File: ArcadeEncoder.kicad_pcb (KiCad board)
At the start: 2 copper layers, 56.6 x 38.7 mm, 7 parts, among them J2 DB9_Male, U1 ProMicro

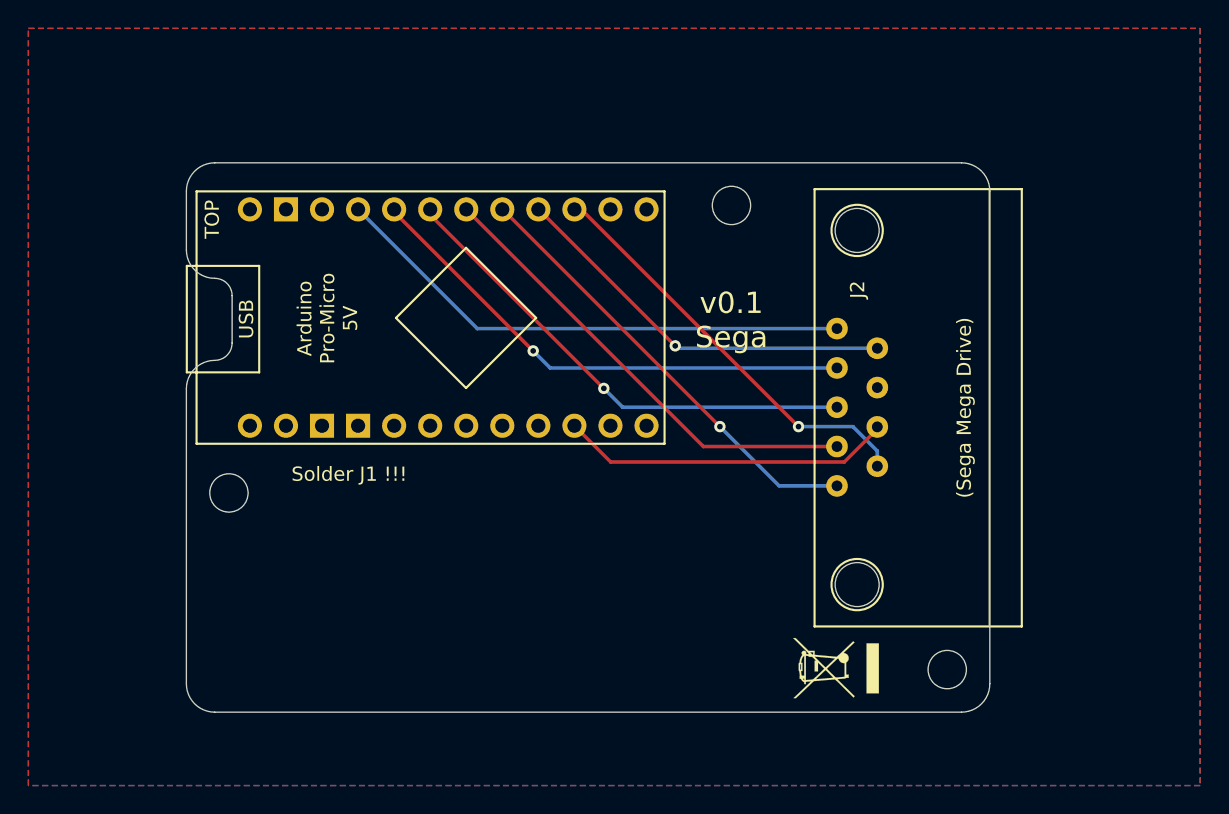
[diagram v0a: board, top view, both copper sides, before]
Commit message: Updated to KiCad 6
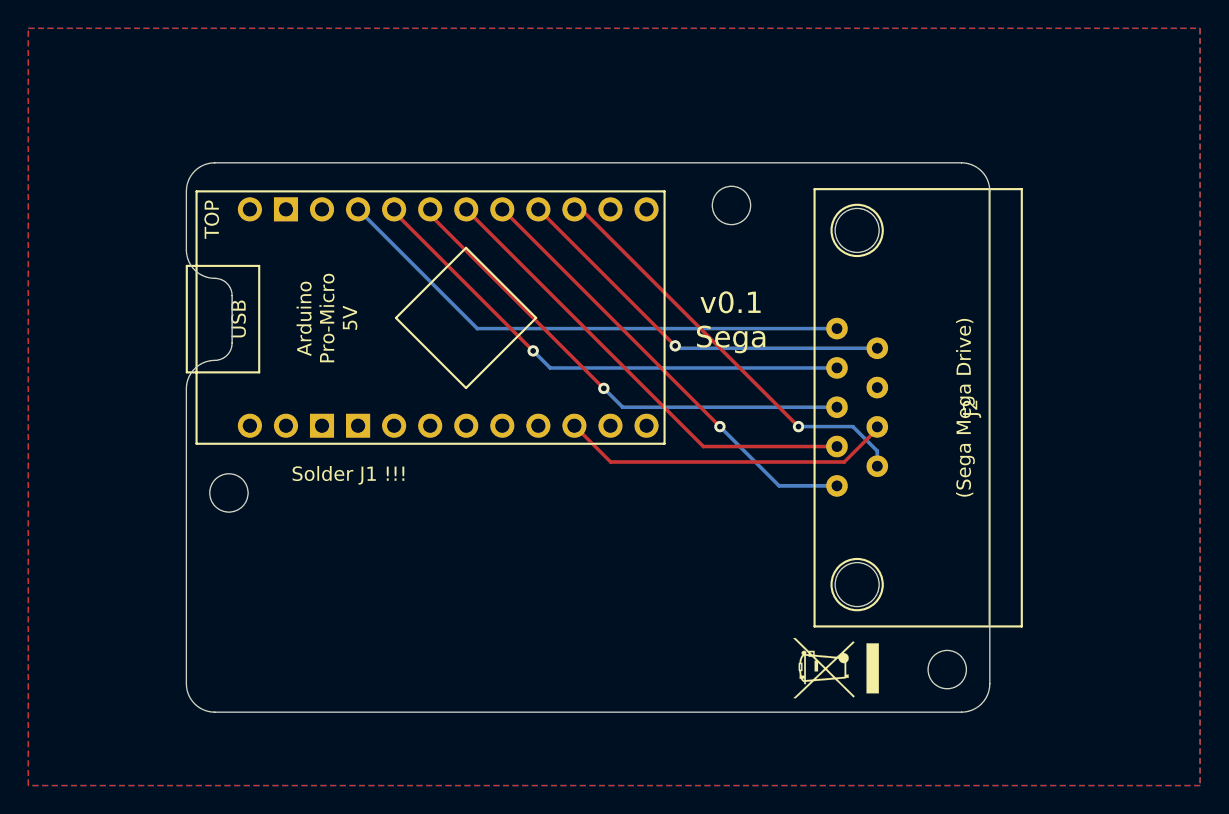
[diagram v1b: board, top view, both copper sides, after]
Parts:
- J2: footprint halibs:D-Sub_Connector_9P-Male -> haus-automatisierung:D-Sub_Connector_9P-Male
- U1: footprint halibs:ArduinoProMicro -> haus-automatisierung:ArduinoProMicro
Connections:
- U1 pad 1: Net-(U1-Pad1) -> unconnected-(U1-Pad1)
- U1 pad 11: Net-(U1-Pad11) -> unconnected-(U1-Pad11)
- U1 pad 12: Net-(U1-Pad12) -> unconnected-(U1-Pad12)
- U1 pad 13: Net-(U1-Pad13) -> unconnected-(U1-Pad13)
- U1 pad 14: Net-(U1-Pad14) -> unconnected-(U1-Pad14)
- U1 pad 2: Net-(U1-Pad2) -> unconnected-(U1-Pad2)
- U1 pad 22: Net-(U1-Pad22) -> unconnected-(U1-Pad22)
- U1 pad 24: Net-(U1-Pad24) -> unconnected-(U1-Pad24)
- U1 pad 5: Net-(U1-Pad5) -> unconnected-(U1-Pad5)
- U1 pad 6: Net-(U1-Pad6) -> unconnected-(U1-Pad6)
- U1 pad 7: Net-(U1-Pad7) -> unconnected-(U1-Pad7)
- U1 pad 8: Net-(U1-Pad8) -> unconnected-(U1-Pad8)
- U1 pad 9: Net-(U1-Pad9) -> unconnected-(U1-Pad9)
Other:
- net class Default removed
